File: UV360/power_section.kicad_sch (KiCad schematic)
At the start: 25 parts, among them J1 5V, J15 5V-SW, J16 12V-SW, J2 12V-IN, J3 12V-OUT

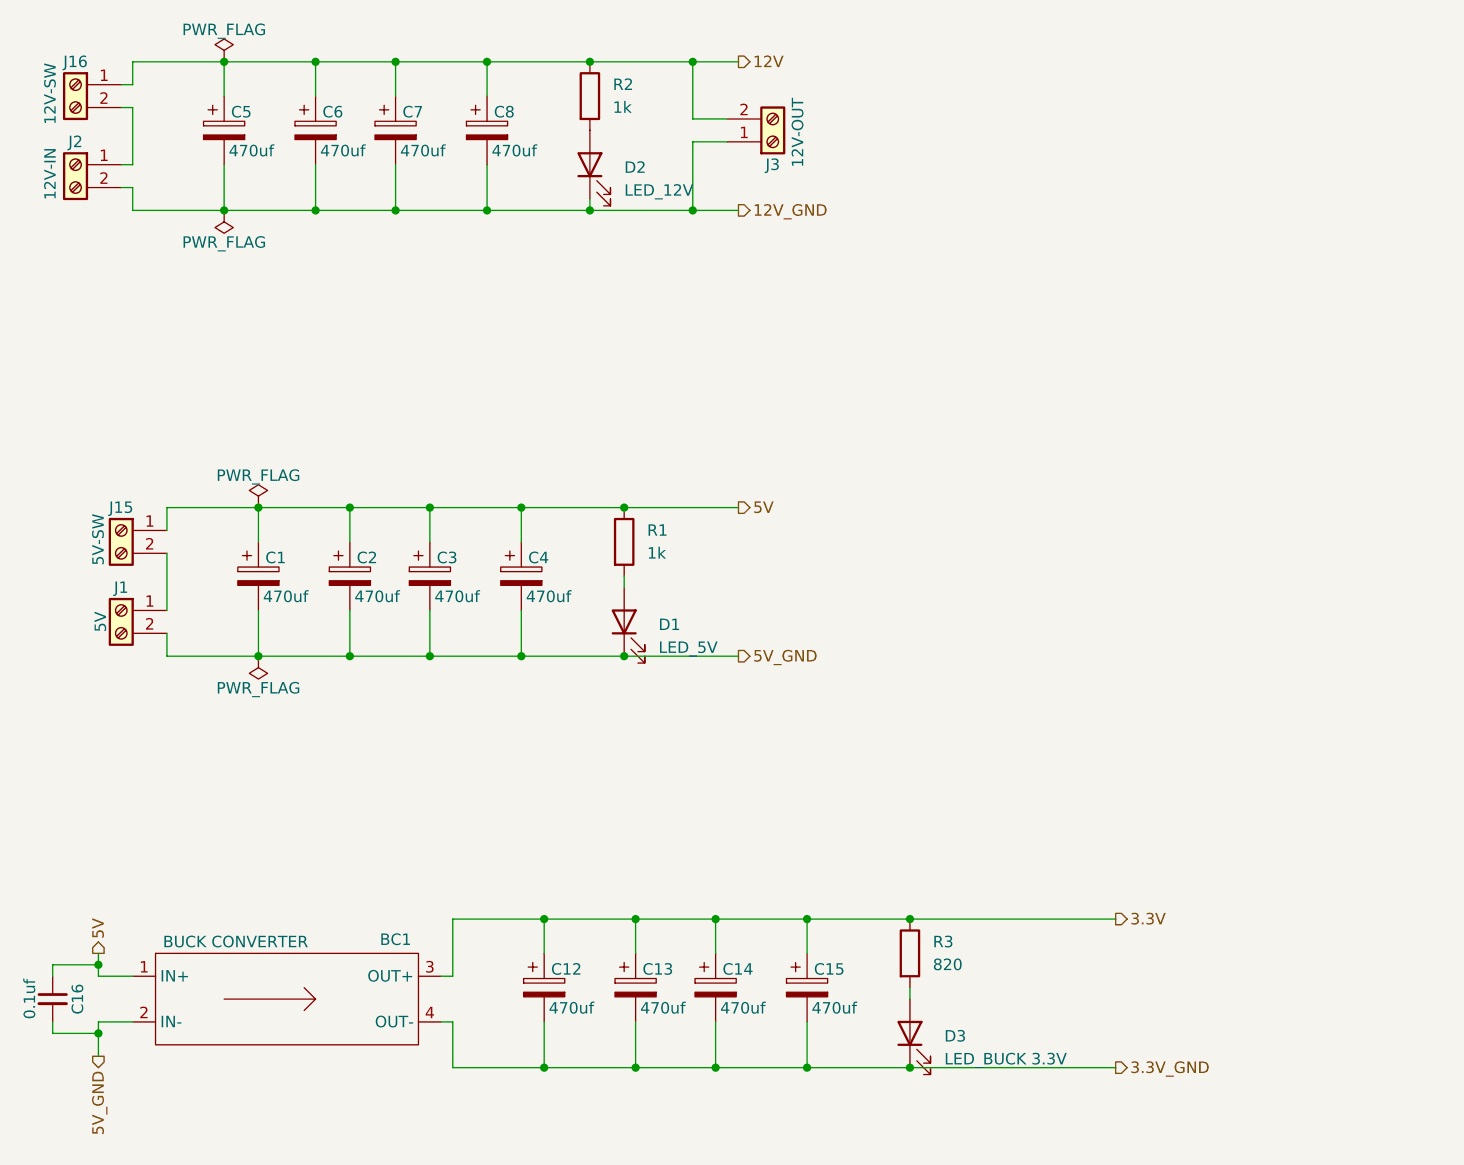
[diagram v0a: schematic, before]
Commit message: power section
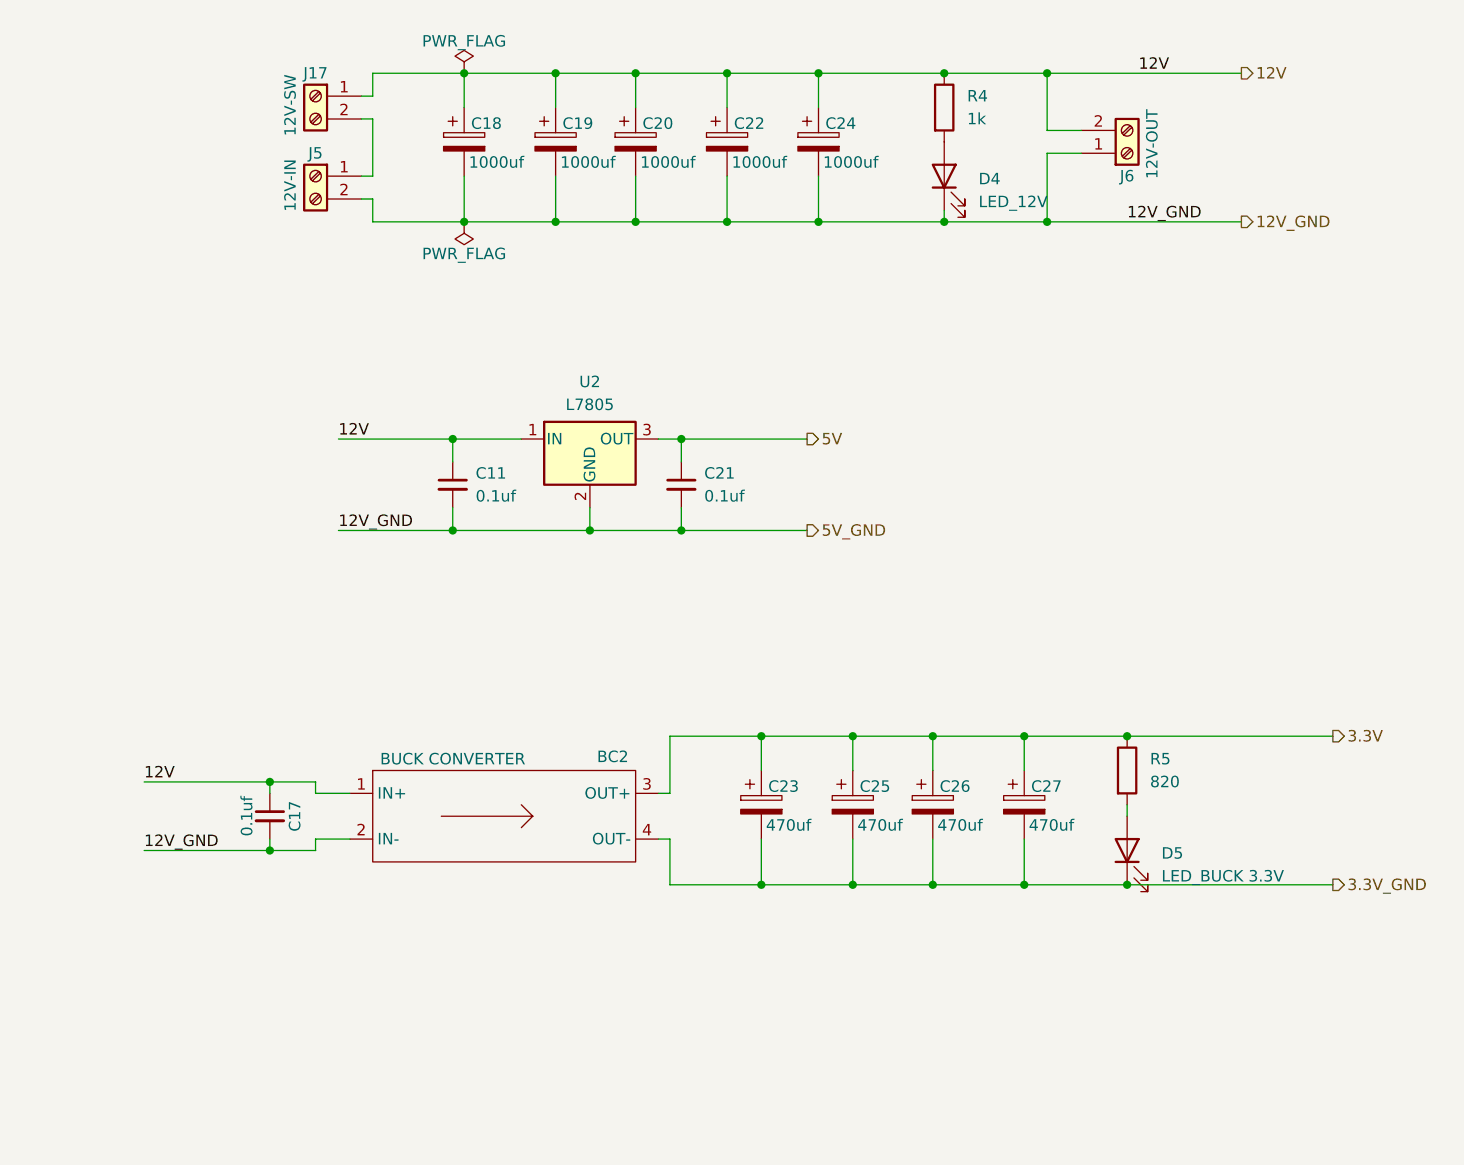
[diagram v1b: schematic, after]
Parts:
- removed BC1: BUCK CONVERTER, Aruns:BUCK CONVERTER, symbol Aruns:BUCK_CONVERTER
- removed C1, C12, C13, C14, C15, C2, C3, C4, C5, C6, C7, C8: 470uf, Capacitor_THT:CP_Radial_D10.0mm_P7.50mm, symbol Device:C_Polarized
- removed C16: 0.1uf, Capacitor_THT:C_Disc_D3.8mm_W2.6mm_P2.50mm, symbol Device:C_Small
- removed D1: LED_5V, LED_THT:LED_D3.0mm, symbol Device:LED
- removed D2: LED_12V, LED_THT:LED_D3.0mm, symbol Device:LED
- removed D3: LED_BUCK 3.3V, LED_THT:LED_D3.0mm, symbol Device:LED
- removed J1: 5V, TerminalBlock_Phoenix:TerminalBlock_Phoenix_MKDS-1,5-2-5.08_1x02_P5.08mm_Horizontal, symbol Connector:Screw_Terminal_01x02
- removed J15: 5V-SW, TerminalBlock_Phoenix:TerminalBlock_Phoenix_MKDS-1,5-2-5.08_1x02_P5.08mm_Horizontal, symbol Connector:Screw_Terminal_01x02
- removed J16: 12V-SW, TerminalBlock_Phoenix:TerminalBlock_Phoenix_MKDS-1,5-2-5.08_1x02_P5.08mm_Horizontal, symbol Connector:Screw_Terminal_01x02
- removed J2: 12V-IN, TerminalBlock_Phoenix:TerminalBlock_Phoenix_MKDS-1,5-2-5.08_1x02_P5.08mm_Horizontal, symbol Connector:Screw_Terminal_01x02
- removed J3: 12V-OUT, TerminalBlock_Phoenix:TerminalBlock_Phoenix_MKDS-1,5-2-5.08_1x02_P5.08mm_Horizontal, symbol Connector:Screw_Terminal_01x02
- removed R1, R2: 1k, Resistor_THT:R_Axial_DIN0204_L3.6mm_D1.6mm_P7.62mm_Horizontal, symbol Device:R
- removed R3: 820, Resistor_THT:R_Axial_DIN0204_L3.6mm_D1.6mm_P7.62mm_Horizontal, symbol Device:R
- added BC2: BUCK CONVERTER, Aruns:BUCK CONVERTER, symbol Aruns:BUCK_CONVERTER
- added C11, C21: 0.1uf, symbol Device:C_Small
- added C17: 0.1uf, Capacitor_THT:C_Disc_D3.8mm_W2.6mm_P2.50mm, symbol Device:C_Small
- added C18, C19, C20, C22, C24: 1000uf, Capacitor_THT:CP_Radial_D10.0mm_P7.50mm, symbol Device:C_Polarized
- added C23, C25, C26, C27: 470uf, Capacitor_THT:CP_Radial_D10.0mm_P7.50mm, symbol Device:C_Polarized
- added D4: LED_12V, LED_THT:LED_D3.0mm, symbol Device:LED
- added D5: LED_BUCK 3.3V, LED_THT:LED_D3.0mm, symbol Device:LED
- added J17: 12V-SW, TerminalBlock_Phoenix:TerminalBlock_Phoenix_MKDS-1,5-2-5.08_1x02_P5.08mm_Horizontal, symbol Connector:Screw_Terminal_01x02
- added J5: 12V-IN, TerminalBlock_Phoenix:TerminalBlock_Phoenix_MKDS-1,5-2-5.08_1x02_P5.08mm_Horizontal, symbol Connector:Screw_Terminal_01x02
- added J6: 12V-OUT, TerminalBlock_Phoenix:TerminalBlock_Phoenix_MKDS-1,5-2-5.08_1x02_P5.08mm_Horizontal, symbol Connector:Screw_Terminal_01x02
- added R4: 1k, Resistor_THT:R_Axial_DIN0204_L3.6mm_D1.6mm_P7.62mm_Horizontal, symbol Device:R
- added R5: 820, Resistor_THT:R_Axial_DIN0204_L3.6mm_D1.6mm_P7.62mm_Horizontal, symbol Device:R
- added U2: L7805, symbol Regulator_Linear:L7805
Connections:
- net 12V: now also BC2.1 (IN+), C11.1, C17.1, C18.1, C19.1, C20.1, C22.1, C24.1, J17.1 (Pin_1), J6.2 (Pin_2), R4.1, U2.1 (IN)
- net 12V_GND: now also BC2.2 (IN-), C11.2, C17.2, C18.2, C19.2, C20.2, C21.2, C22.2, C24.2, D4.1 (K), J5.2 (Pin_2), J6.1 (Pin_1), U2.2 (GND)
- net 3.3V: now also BC2.3 (OUT+), C23.1, C25.1, C26.1, C27.1, R5.1
- net 3.3V_GND: now also BC2.4 (OUT-), C23.2, C25.2, C26.2, C27.2, D5.1 (K)
- net 5V: now also C21.1, U2.3 (OUT)
- new net: D5.2 (A), R5.2
- new net: J17.2 (Pin_2), J5.1 (Pin_1)
- new net: D4.2 (A), R4.2
